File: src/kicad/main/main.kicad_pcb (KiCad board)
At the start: 4 copper layers, 50 x 50 mm, 108 parts

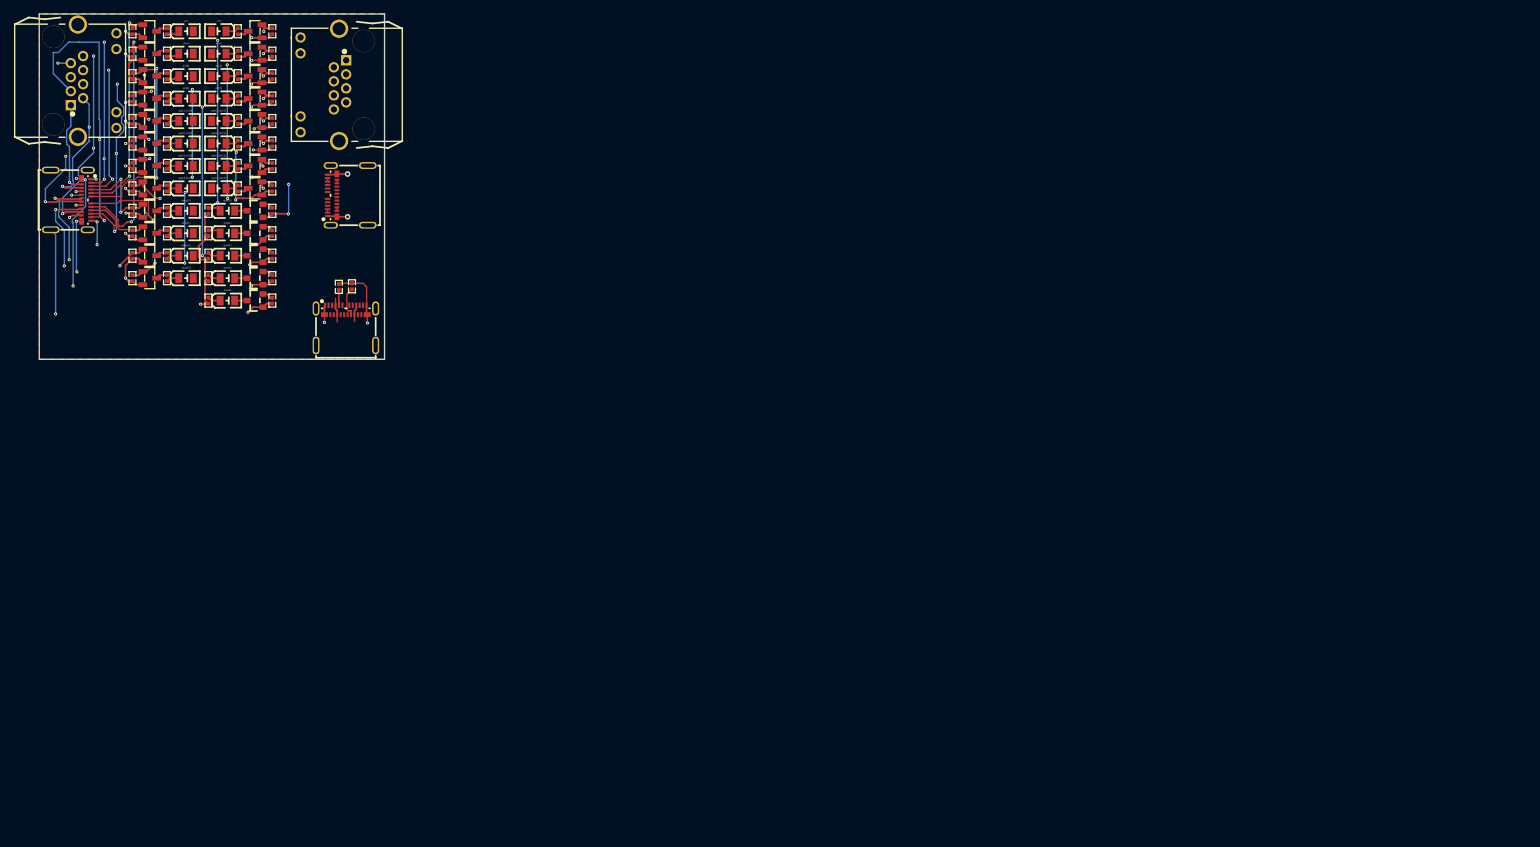
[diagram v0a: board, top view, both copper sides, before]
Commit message: Add components
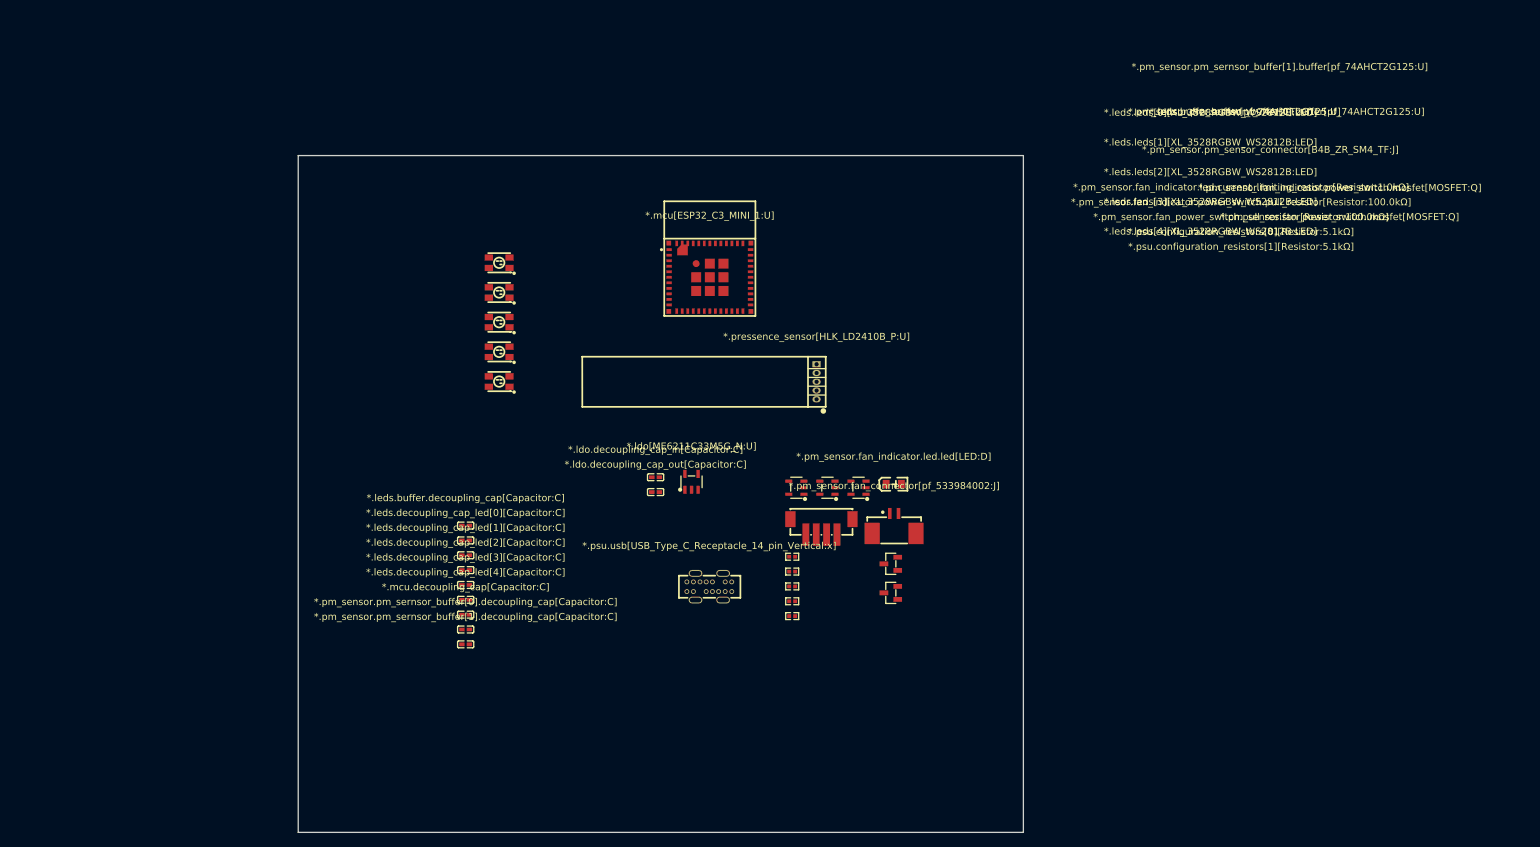
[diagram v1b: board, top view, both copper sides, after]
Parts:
- removed G***: Made with faebryk, logo:faebryk_logo
- removed psu.configuration_resistors[0][Resistor:5.0KΩ], psu.configuration_resistors[1][Resistor:5.0KΩ]: 5.0KΩ, lcsc:R0402
- removed psu.usb[USB_C_Receptacle:x], tester.usb_c[0][USB_C_Receptacle:x], tester.usb_c[1][USB_C_Receptacle:x]: x, lcsc:USB-C-SMD_TYPE-C-USB-18
- removed tester.cc1.indicator.led.current_limiting_resistor[Resistor:1KΩ], tester.cc2.indicator.led.current_limiting_resistor[Resistor:1KΩ], tester.d1[0].indicator.led.current_limiting_resistor[Resistor:1KΩ], tester.d1[1].indicator.led.current_limiting_resistor[Resistor:1KΩ], tester.d2[0].indicator.led.current_limiting_resistor[Resistor:1KΩ], tester.d2[1].indicator.led.current_limiting_resistor[Resistor:1KΩ], tester.gnd[0].indicator.led.current_limiting_resistor[Resistor:1KΩ], tester.gnd[1].indicator.led.current_limiting_resistor[Resistor:1KΩ], tester.gnd[2].indicator.led.current_limiting_resistor[Resistor:1KΩ], tester.gnd[3].indicator.led.current_limiting_resistor[Resistor:1KΩ], tester.pair1_rx1[0].indicator.led.current_limiting_resistor[Resistor:1KΩ], tester.pair1_rx1[1].indicator.led.current_limiting_resistor[Resistor:1KΩ], tester.pair2_rx2[0].indicator.led.current_limiting_resistor[Resistor:1KΩ], tester.pair2_rx2[1].indicator.led.current_limiting_resistor[Resistor:1KΩ], tester.pair3_tx1[0].indicator.led.current_limiting_resistor[Resistor:1KΩ], tester.pair3_tx1[1].indicator.led.current_limiting_resistor[Resistor:1KΩ], tester.pair4_tx2[0].indicator.led.current_limiting_resistor[Resistor:1KΩ], tester.pair4_tx2[1].indicator.led.current_limiting_resistor[Resistor:1KΩ], tester.sbu1.indicator.led.current_limiting_resistor[Resistor:1KΩ], tester.sbu2.indicator.led.current_limiting_resistor[Resistor:1KΩ], tester.shield.indicator.led.current_limiting_resistor[Resistor:1KΩ], tester.vbus[0].indicator.led.current_limiting_resistor[Resistor:1KΩ], tester.vbus[1].indicator.led.current_limiting_resistor[Resistor:1KΩ], tester.vbus[2].indicator.led.current_limiting_resistor[Resistor:1KΩ], tester.vbus[3].indicator.led.current_limiting_resistor[Resistor:1KΩ]: 1KΩ, lcsc:R0402
- removed tester.cc1.indicator.led.led[LED:D], tester.cc2.indicator.led.led[LED:D], tester.d1[0].indicator.led.led[LED:D], tester.d1[1].indicator.led.led[LED:D], tester.d2[0].indicator.led.led[LED:D], tester.d2[1].indicator.led.led[LED:D], tester.gnd[0].indicator.led.led[LED:D], tester.gnd[1].indicator.led.led[LED:D], tester.gnd[2].indicator.led.led[LED:D], tester.gnd[3].indicator.led.led[LED:D], tester.pair1_rx1[0].indicator.led.led[LED:D], tester.pair1_rx1[1].indicator.led.led[LED:D], tester.pair2_rx2[0].indicator.led.led[LED:D], tester.pair2_rx2[1].indicator.led.led[LED:D], tester.pair3_tx1[0].indicator.led.led[LED:D], tester.pair3_tx1[1].indicator.led.led[LED:D], tester.pair4_tx2[0].indicator.led.led[LED:D], tester.pair4_tx2[1].indicator.led.led[LED:D], tester.sbu1.indicator.led.led[LED:D], tester.sbu2.indicator.led.led[LED:D], tester.shield.indicator.led.led[LED:D], tester.vbus[0].indicator.led.led[LED:D], tester.vbus[1].indicator.led.led[LED:D], tester.vbus[2].indicator.led.led[LED:D], tester.vbus[3].indicator.led.led[LED:D]: D, lcsc:LED0805-R-RD
- removed tester.cc1.indicator.power_switch.mosfet[MOSFET:Q], tester.cc2.indicator.power_switch.mosfet[MOSFET:Q], tester.d1[0].indicator.power_switch.mosfet[MOSFET:Q], tester.d1[1].indicator.power_switch.mosfet[MOSFET:Q], tester.d2[0].indicator.power_switch.mosfet[MOSFET:Q], tester.d2[1].indicator.power_switch.mosfet[MOSFET:Q], tester.pair1_rx1[0].indicator.power_switch.mosfet[MOSFET:Q], tester.pair1_rx1[1].indicator.power_switch.mosfet[MOSFET:Q], tester.pair2_rx2[0].indicator.power_switch.mosfet[MOSFET:Q], tester.pair2_rx2[1].indicator.power_switch.mosfet[MOSFET:Q], tester.pair3_tx1[0].indicator.power_switch.mosfet[MOSFET:Q], tester.pair3_tx1[1].indicator.power_switch.mosfet[MOSFET:Q], tester.pair4_tx2[0].indicator.power_switch.mosfet[MOSFET:Q], tester.pair4_tx2[1].indicator.power_switch.mosfet[MOSFET:Q], tester.sbu1.indicator.power_switch.mosfet[MOSFET:Q], tester.sbu2.indicator.power_switch.mosfet[MOSFET:Q], tester.vbus[0].indicator.power_switch.mosfet[MOSFET:Q], tester.vbus[1].indicator.power_switch.mosfet[MOSFET:Q], tester.vbus[2].indicator.power_switch.mosfet[MOSFET:Q], tester.vbus[3].indicator.power_switch.mosfet[MOSFET:Q]: Q, lcsc:SOT-23-3_L2.9-W1.3-P1.90-LS2.4-BR
- removed tester.cc1.indicator.power_switch.pull_resistor[Resistor:100KΩ], tester.cc2.indicator.power_switch.pull_resistor[Resistor:100KΩ], tester.d1[0].indicator.power_switch.pull_resistor[Resistor:100KΩ], tester.d1[1].indicator.power_switch.pull_resistor[Resistor:100KΩ], tester.d2[0].indicator.power_switch.pull_resistor[Resistor:100KΩ], tester.d2[1].indicator.power_switch.pull_resistor[Resistor:100KΩ], tester.gnd[0].indicator.power_switch.pull_resistor[Resistor:100KΩ], tester.gnd[1].indicator.power_switch.pull_resistor[Resistor:100KΩ], tester.gnd[2].indicator.power_switch.pull_resistor[Resistor:100KΩ], tester.gnd[3].indicator.power_switch.pull_resistor[Resistor:100KΩ], tester.pair1_rx1[0].indicator.power_switch.pull_resistor[Resistor:100KΩ], tester.pair1_rx1[1].indicator.power_switch.pull_resistor[Resistor:100KΩ], tester.pair2_rx2[0].indicator.power_switch.pull_resistor[Resistor:100KΩ], tester.pair2_rx2[1].indicator.power_switch.pull_resistor[Resistor:100KΩ], tester.pair3_tx1[0].indicator.power_switch.pull_resistor[Resistor:100KΩ], tester.pair3_tx1[1].indicator.power_switch.pull_resistor[Resistor:100KΩ], tester.pair4_tx2[0].indicator.power_switch.pull_resistor[Resistor:100KΩ], tester.pair4_tx2[1].indicator.power_switch.pull_resistor[Resistor:100KΩ], tester.sbu1.indicator.power_switch.pull_resistor[Resistor:100KΩ], tester.sbu2.indicator.power_switch.pull_resistor[Resistor:100KΩ], tester.shield.indicator.power_switch.pull_resistor[Resistor:100KΩ], tester.vbus[0].indicator.power_switch.pull_resistor[Resistor:100KΩ], tester.vbus[1].indicator.power_switch.pull_resistor[Resistor:100KΩ], tester.vbus[2].indicator.power_switch.pull_resistor[Resistor:100KΩ], tester.vbus[3].indicator.power_switch.pull_resistor[Resistor:100KΩ]: 100KΩ, lcsc:R0402
- removed tester.gnd[0].indicator.power_switch.mosfet[MOSFET:Q], tester.gnd[1].indicator.power_switch.mosfet[MOSFET:Q], tester.gnd[2].indicator.power_switch.mosfet[MOSFET:Q], tester.gnd[3].indicator.power_switch.mosfet[MOSFET:Q], tester.shield.indicator.power_switch.mosfet[MOSFET:Q]: Q, lcsc:SOT-23_L2.9-W1.3-P1.90-LS2.4-BR
- removed tester.rj45[0][RJ45_Receptacle:x], tester.rj45[1][RJ45_Receptacle:x]: x, lcsc:RJ45-TH_B-1-1
- added *.ldo.decoupling_cap_in[Capacitor:C]: C, lcsc:C0402, F.Cu at (89.2, 67.1)
- added *.ldo.decoupling_cap_out[Capacitor:C]: C, lcsc:C0402, F.Cu at (89.2, 69.2)
- added *.ldo[ME6211C33M5G_N:U]: U, lcsc:SOT-23-5_L3.0-W1.7-P0.95-LS2.8-BL, F.Cu at (94.5, 67.7)
- added *.leds.buffer.buffer[pf_74AHCT2G125:U]: U, lcsc:SC-74A-5_L2.9-W1.6-P0.95-LS2.8-BR, F.Cu at (109.6, 68.6)
- added *.leds.buffer.decoupling_cap[Capacitor:C]: C, lcsc:C0402, F.Cu at (61.7, 74.1)
- added *.leds.decoupling_cap_led[0][Capacitor:C]: C, lcsc:C0402, F.Cu at (61.7, 76.2)
- added *.leds.decoupling_cap_led[1][Capacitor:C]: C, lcsc:C0402, F.Cu at (61.7, 78.4)
- added *.leds.decoupling_cap_led[2][Capacitor:C]: C, lcsc:C0402, F.Cu at (61.7, 80.5)
- added *.leds.decoupling_cap_led[3][Capacitor:C]: C, lcsc:C0402, F.Cu at (61.7, 82.7)
- added *.leds.decoupling_cap_led[4][Capacitor:C]: C, lcsc:C0402, F.Cu at (61.7, 84.8)
- added *.leds.leds[0][XL_3528RGBW_WS2812B:LED]: LED, lcsc:LED-SMD_4P-L3.5-W2.8-BR-1, F.Cu at (66.6, 36.0)
- added *.leds.leds[1][XL_3528RGBW_WS2812B:LED]: LED, lcsc:LED-SMD_4P-L3.5-W2.8-BR-1, F.Cu at (66.6, 40.3)
- added *.leds.leds[2][XL_3528RGBW_WS2812B:LED]: LED, lcsc:LED-SMD_4P-L3.5-W2.8-BR-1, F.Cu at (66.6, 44.6)
- added *.leds.leds[3][XL_3528RGBW_WS2812B:LED]: LED, lcsc:LED-SMD_4P-L3.5-W2.8-BR-1, F.Cu at (66.6, 48.9)
- added *.leds.leds[4][XL_3528RGBW_WS2812B:LED]: LED, lcsc:LED-SMD_4P-L3.5-W2.8-BR-1, F.Cu at (66.6, 53.2)
- added *.mcu.decoupling_cap[Capacitor:C]: C, lcsc:C0402, F.Cu at (61.7, 87.0)
- added *.mcu[ESP32_C3_MINI_1:U]: U, lcsc:WIFIM-SMD_ESP32-C3-MINI-1, F.Cu at (97.1, 38.1)
- added *.pm_sensor.fan_connector[pf_533984002:J]: J, lcsc:CONN-SMD_1.25-2P, F.Cu at (123.8, 73.8)
- added *.pm_sensor.fan_indicator.led.current_limiting_resistor[Resistor:1.0kΩ]: 1.0kΩ, lcsc:R0402, F.Cu at (109.0, 78.6)
- added *.pm_sensor.fan_indicator.led.led[LED:D]: D, lcsc:LED0805-RD_RED, F.Cu at (123.7, 68.1)
- added *.pm_sensor.fan_indicator.power_switch.mosfet[MOSFET:Q]: Q, lcsc:SOT-23-3_L2.9-W1.3-P1.90-LS2.4-BR, F.Cu at (123.3, 79.6)
- added *.pm_sensor.fan_indicator.power_switch.pull_resistor[Resistor:100.0kΩ]: 100.0kΩ, lcsc:R0402, F.Cu at (109.0, 80.7)
- added *.pm_sensor.fan_power_switch.mosfet[MOSFET:Q]: Q, lcsc:SOT-23-3_L2.9-W1.3-P1.90-LS2.4-BR, F.Cu at (123.3, 83.8)
- added *.pm_sensor.fan_power_switch.pull_resistor[Resistor:100.0kΩ]: 100.0kΩ, lcsc:R0402, F.Cu at (109.0, 82.9)
- added *.pm_sensor.pm_sensor_connector[B4B_ZR_SM4_TF:J]: J, lcsc:CONN-SMD_ZH1.5-4AB, F.Cu at (113.3, 74.3)
- added *.pm_sensor.pm_sernsor_buffer[0].buffer[pf_74AHCT2G125:U]: U, lcsc:SC-74A-5_L2.9-W1.6-P0.95-LS2.8-BR, F.Cu at (114.1, 68.6)
- added *.pm_sensor.pm_sernsor_buffer[0].decoupling_cap[Capacitor:C]: C, lcsc:C0402, F.Cu at (61.7, 89.1)
- added *.pm_sensor.pm_sernsor_buffer[1].buffer[pf_74AHCT2G125:U]: U, lcsc:SC-74A-5_L2.9-W1.6-P0.95-LS2.8-BR, F.Cu at (118.6, 68.6)
- added *.pm_sensor.pm_sernsor_buffer[1].decoupling_cap[Capacitor:C]: C, lcsc:C0402, F.Cu at (61.7, 91.3)
- added *.pressence_sensor[HLK_LD2410B_P:U]: U, lcsc:SENSORM-TH_HLK-LD2410B-P, F.Cu at (112.6, 53.3)
- added *.psu.configuration_resistors[0][Resistor:5.1kΩ]: 5.1kΩ, lcsc:R0402, F.Cu at (109.0, 85.0)
- added *.psu.configuration_resistors[1][Resistor:5.1kΩ]: 5.1kΩ, lcsc:R0402, F.Cu at (109.0, 87.2)
- added *.psu.usb[USB_Type_C_Receptacle_14_pin_Vertical:x]: x, lcsc:USB-C-TH_TYPE-C-USB-14P, F.Cu at (97.0, 82.9)
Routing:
- net tester.vbus[1].indicator[LEDIndicator:virt]:3-tester.shield.indicator[LEDIndicator:virt]:3-tester.gn: track 245.9 -> 0.00 mm, vias 23 -> 0
- net tester.d2[1][PairTester:virt]:4-tester.d2[1].indicator[LEDIndicator:virt]-tester.d2[1].indicator.pow: track 65.7 -> 0.00 mm, vias 5 -> 0
- net tester.shield.indicator.power_switch[PowerSwitch:virt]-tester.shield.indicator[LEDIndicator:virt]-te: track 63.8 -> 0.00 mm, vias 2 -> 0
- net tester.pair4_tx2[1].indicator[LEDIndicator:virt]-tester.pair4_tx2[1].indicator.power_switch[PowerSwi: track 62.8 -> 0.00 mm, vias 5 -> 0
- net tester.pair2_rx2[1].indicator.power_switch[PowerSwitch:virt]-tester.pair2_rx2[1].indicator[LEDIndica: track 55.9 -> 0.00 mm, vias 4 -> 0
- net tester.d2[0][PairTester:virt]:4-tester.d2[0].indicator.power_switch[PowerSwitch:virt]-tester.d2[0].i: track 54.5 -> 0.00 mm, vias 5 -> 0
- net tester.cc2.indicator.power_switch[PowerSwitch:virt]-tester.cc2.indicator[LEDIndicator:virt]-tester.c: track 53.5 -> 0.00 mm, vias 4 -> 0
- net tester.d1[1].indicator.power_switch[PowerSwitch:virt]-tester.d1[1][PairTester:virt]:4-tester.d1[1].i: track 52.5 -> 0.00 mm, vias 3 -> 0
- net tester.pair2_rx2[0].indicator[LEDIndicator:virt]-tester.pair2_rx2[0][PairTester:virt]:4-tester.pair2: track 52.0 -> 0.00 mm, vias 3 -> 0
- net tester.sbu2.indicator.power_switch[PowerSwitch:virt]-tester.sbu2[PairTester:virt]:4-tester.sbu2.indi: track 51.2 -> 0.00 mm, vias 4 -> 0
- net tester.pair3_tx1[1].indicator[LEDIndicator:virt]-tester.pair3_tx1[1][PairTester:virt]:4-tester.pair3: track 48.1 -> 0.00 mm, vias 3 -> 0
- net tester.pair4_tx2[0].indicator[LEDIndicator:virt]-tester.pair4_tx2[0].indicator.power_switch[PowerSwi: track 47.5 -> 0.00 mm, vias 3 -> 0
- net tester.gnd[3][PairTester:virt]:4-tester.gnd[3].indicator[LEDIndicator:virt]-tester.gnd[3].indicator.: track 47.5 -> 0.00 mm, vias 4 -> 0
- net tester.pair1_rx1[1][PairTester:virt]:4-tester.pair1_rx1[1].indicator[LEDIndicator:virt]-tester.pair1: track 45.9 -> 0.00 mm, vias 3 -> 0
- net tester.pair3_tx1[0].indicator.power_switch[PowerSwitch:virt]-tester.pair3_tx1[0][PairTester:virt]:4-: track 42.5 -> 0.00 mm, vias 4 -> 0
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- removed copper zone on F.Cu, net tester.pair1_rx1[1].indicator.led[PoweredLED:virt]-tester.d2[1].indicator.power_switch[PowerSwitch:v
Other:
- board size 50 x 50 mm -> 105 x 98 mm
- copper layers 4 -> 2
- board text removed: "USB-C CableTester v1.0.1 https://github.com/IoannisP-ITENG/CableTester"
- board text removed: "cc1"
- board text removed: "cc2"
- board text removed: "d1[0]"
- board text removed: "d1[1]"
- board text removed: "d2[0]"
- board text removed: "d2[1]"
- board text removed: "gnd[0]"
- board text removed: "gnd[1]"
- board text removed: "gnd[2]"
- board text removed: "gnd[3]"
- board text removed: "pair1_rx1[0]"
- board text removed: "pair1_rx1[1]"
- board text removed: "pair2_rx2[0]"
- board text removed: "pair2_rx2[1]"
- board text removed: "pair3_tx1[0]"
- board text removed: "pair3_tx1[1]"
- board text removed: "pair4_tx2[0]"
- board text removed: "pair4_tx2[1]"
- board text removed: "sbu1"
- board text removed: "sbu2"
- board text removed: "shield"
- board text removed: "vbus[0]"
- board text removed: "vbus[1]"
- board text removed: "vbus[2]"
- board text removed: "vbus[3]"
